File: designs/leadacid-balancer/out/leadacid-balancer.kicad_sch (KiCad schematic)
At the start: 0 parts

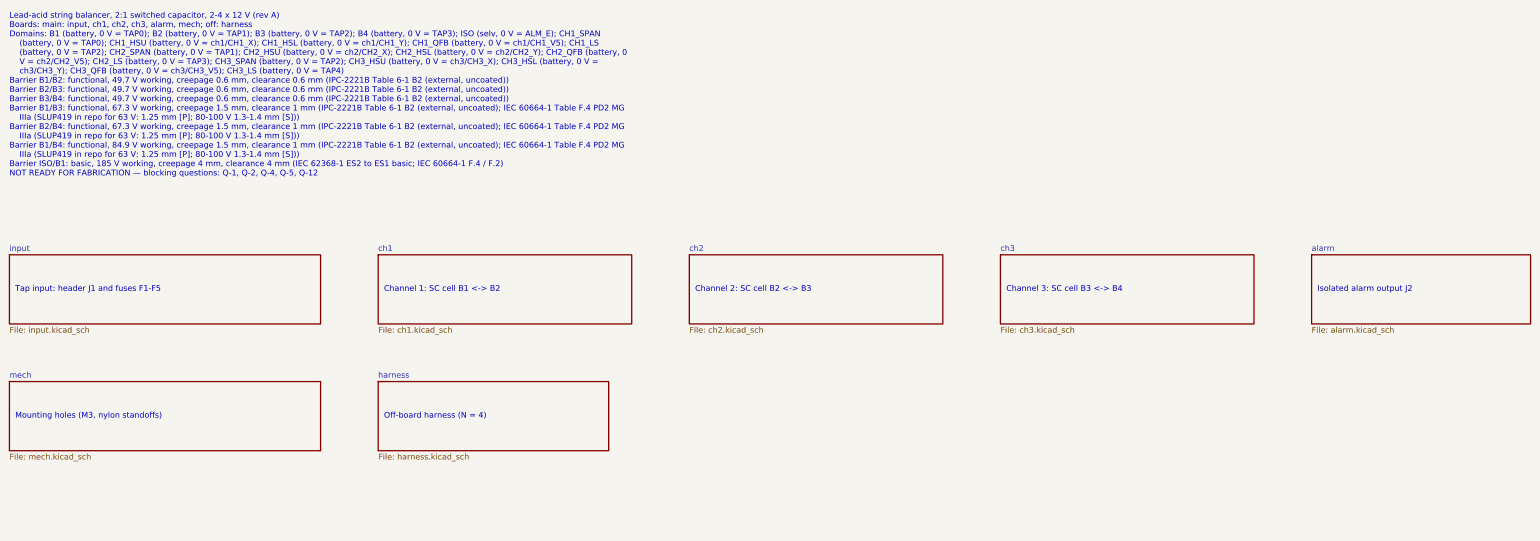
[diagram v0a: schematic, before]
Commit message: designs: work-in-progress (review fixes under way)
Co-Authored-By: Claude Opus 5.5 <noreply@anthropic.com>
Claude-Session: https://claude.ai/code/session_01VFJn9VbX8h27kf4LpLwEtn
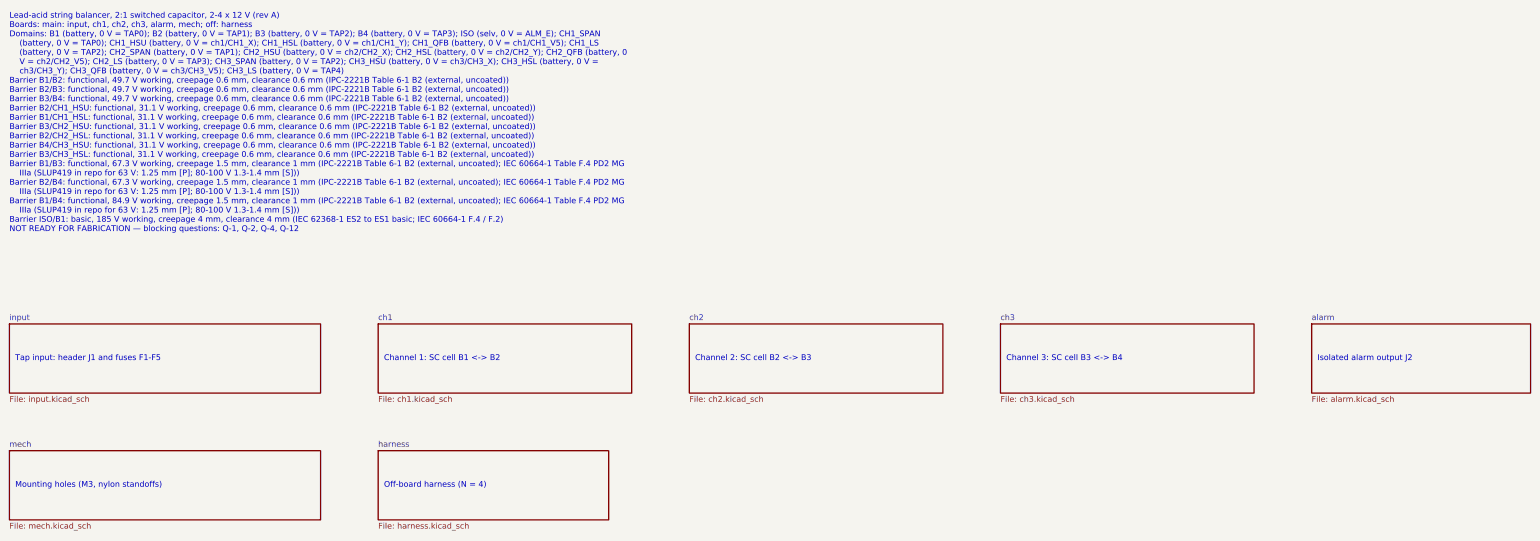
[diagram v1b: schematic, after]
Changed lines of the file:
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@@
 	)
 	(sheet
-		(at 25.4 78.74)
+		(at 25.4 93.98)
 		(size 68.58 15.24)
 		(exclude_from_sim no)
@@
 		)
 		(property "Sheetname" "input"
-			(at 25.4 78.04 0)
+			(at 25.4 93.28 0)
 			(effects
 				(font (size 1.27 1.27))
@@
 		)
 		(property "Sheetfile" "input.kicad_sch"
-			(at 25.4 94.58 0)
+			(at 25.4 109.82 0)
 			(effects
 				(font (size 1.27 1.27))
@@
 	(text "Tap input: header J1 and fuses F1-F5"
 		(exclude_from_sim no)
-		(at 26.67 86.36 0)
-		(effects
-			(font (size 1.27 1.27))
-			(justify left)
-		)
-	)
-	(sheet
-		(at 106.68 78.74)
+		(at 26.67 101.6 0)
+		(effects
+			(font (size 1.27 1.27))
+			(justify left)
+		)
+	)
+	(sheet
+		(at 106.68 93.98)
 		(size 55.88 15.24)
 		(exclude_from_sim no)
@@
 		)
 		(property "Sheetname" "ch1"
-			(at 106.68 78.04 0)
+			(at 106.68 93.28 0)
 			(effects
 				(font (size 1.27 1.27))
@@
 		)
 		(property "Sheetfile" "ch1.kicad_sch"
-			(at 106.68 94.58 0)
+			(at 106.68 109.82 0)
 			(effects
 				(font (size 1.27 1.27))
@@
 	(text "Channel 1: SC cell B1 <-> B2"
 		(exclude_from_sim no)
-		(at 107.95 86.36 0)
-		(effects
-			(font (size 1.27 1.27))
-			(justify left)
-		)
-	)
-	(sheet
-		(at 175.26 78.74)
+		(at 107.95 101.6 0)
+		(effects
+			(font (size 1.27 1.27))
+			(justify left)
+		)
+	)
+	(sheet
+		(at 175.26 93.98)
 		(size 55.88 15.24)
 		(exclude_from_sim no)
@@
 		)
 		(property "Sheetname" "ch2"
-			(at 175.26 78.04 0)
+			(at 175.26 93.28 0)
 			(effects
 				(font (size 1.27 1.27))
@@
 		)
 		(property "Sheetfile" "ch2.kicad_sch"
-			(at 175.26 94.58 0)
+			(at 175.26 109.82 0)
 			(effects
 				(font (size 1.27 1.27))
@@
 	(text "Channel 2: SC cell B2 <-> B3"
 		(exclude_from_sim no)
-		(at 176.53 86.36 0)
-		(effects
-			(font (size 1.27 1.27))
-			(justify left)
-		)
-	)
-	(sheet
-		(at 243.84 78.74)
+		(at 176.53 101.6 0)
+		(effects
+			(font (size 1.27 1.27))
+			(justify left)
+		)
+	)
+	(sheet
+		(at 243.84 93.98)
 		(size 55.88 15.24)
 		(exclude_from_sim no)
@@
 		)
 		(property "Sheetname" "ch3"
-			(at 243.84 78.04 0)
+			(at 243.84 93.28 0)
 			(effects
 				(font (size 1.27 1.27))
@@
 		)
 		(property "Sheetfile" "ch3.kicad_sch"
-			(at 243.84 94.58 0)
+			(at 243.84 109.82 0)
 			(effects
 				(font (size 1.27 1.27))
@@
 	(text "Channel 3: SC cell B3 <-> B4"
 		(exclude_from_sim no)
-		(at 245.11 86.36 0)
-		(effects
-			(font (size 1.27 1.27))
-			(justify left)
-		)
-	)
-	(sheet
-		(at 312.42 78.74)
+		(at 245.11 101.6 0)
+		(effects
+			(font (size 1.27 1.27))
+			(justify left)
+		)
+	)
+	(sheet
+		(at 312.42 93.98)
 		(size 48.26 15.24)
 		(exclude_from_sim no)
@@
 		)
 		(property "Sheetname" "alarm"
-			(at 312.42 78.04 0)
+			(at 312.42 93.28 0)
 			(effects
 				(font (size 1.27 1.27))
@@
 		)
 		(property "Sheetfile" "alarm.kicad_sch"
-			(at 312.42 94.58 0)
+			(at 312.42 109.82 0)
 			(effects
 				(font (size 1.27 1.27))
@@
 	(text "Isolated alarm output J2"
 		(exclude_from_sim no)
-		(at 313.69 86.36 0)
-		(effects
-			(font (size 1.27 1.27))
-			(justify left)
-		)
-	)
-	(sheet
-		(at 25.4 106.68)
+		(at 313.69 101.6 0)
+		(effects
+			(font (size 1.27 1.27))
+			(justify left)
+		)
+	)
+	(sheet
+		(at 25.4 121.92)
 		(size 68.58 15.24)
 		(exclude_from_sim no)
@@
 		)
 		(property "Sheetname" "mech"
-			(at 25.4 105.98 0)
+			(at 25.4 121.22 0)
 			(effects
 				(font (size 1.27 1.27))
@@
 		)
 		(property "Sheetfile" "mech.kicad_sch"
-			(at 25.4 122.52 0)
+			(at 25.4 137.76 0)
 			(effects
 				(font (size 1.27 1.27))
@@
 	(text "Mounting holes (M3, nylon standoffs)"
 		(exclude_from_sim no)
-		(at 26.67 114.3 0)
-		(effects
-			(font (size 1.27 1.27))
-			(justify left)
-		)
-	)
-	(sheet
-		(at 106.68 106.68)
+		(at 26.67 129.54 0)
+		(effects
+			(font (size 1.27 1.27))
+			(justify left)
+		)
+	)
+	(sheet
+		(at 106.68 121.92)
 		(size 50.8 15.24)
 		(exclude_from_sim no)
@@
 		)
 		(property "Sheetname" "harness"
-			(at 106.68 105.98 0)
+			(at 106.68 121.22 0)
 			(effects
 				(font (size 1.27 1.27))
@@
 		)
 		(property "Sheetfile" "harness.kicad_sch"
-			(at 106.68 122.52 0)
+			(at 106.68 137.76 0)
 			(effects
 				(font (size 1.27 1.27))
@@
 	(text "Off-board harness (N = 4)"
 		(exclude_from_sim no)
-		(at 107.95 114.3 0)
-		(effects
-			(font (size 1.27 1.27))
-			(justify left)
-		)
-	)
-	(text "Lead-acid string balancer, 2:1 switched capacitor, 2-4 x 12 V (rev A)\nBoards: main: input, ch1, ch2, ch3, alarm, mech; off: harness\nDomains: B1 (battery, 0 V = TAP0); B2 (battery, 0 V = TAP1); B3 (battery, 0 V = TAP2); B4 (battery, 0 V = TAP3); ISO (selv, 0 V = ALM_E); CH1_SPAN\n    (battery, 0 V = TAP0); CH1_HSU (battery, 0 V = ch1/CH1_X); CH1_HSL (battery, 0 V = ch1/CH1_Y); CH1_QFB (battery, 0 V = ch1/CH1_V5); CH1_LS\n    (battery, 0 V = TAP2); CH2_SPAN (battery, 0 V = TAP1); CH2_HSU (battery, 0 V = ch2/CH2_X); CH2_HSL (battery, 0 V = ch2/CH2_Y); CH2_QFB (battery, 0\n    V = ch2/CH2_V5); CH2_LS (battery, 0 V = TAP3); CH3_SPAN (battery, 0 V = TAP2); CH3_HSU (battery, 0 V = ch3/CH3_X); CH3_HSL (battery, 0 V =\n    ch3/CH3_Y); CH3_QFB (battery, 0 V = ch3/CH3_V5); CH3_LS (battery, 0 V = TAP4)\nBarrier B1/B2: functional, 49.7 V working, creepage 0.6 mm, clearance 0.6 mm (IPC-2221B Table 6-1 B2 (external, uncoated))\nBarrier B2/B3: functional, 49.7 V working, creepage 0.6 mm, clearance 0.6 mm (IPC-2221B Table 6-1 B2 (external, uncoated))\nBarrier B3/B4: functional, 49.7 V working, creepage 0.6 mm, clearance 0.6 mm (IPC-2221B Table 6-1 B2 (external, uncoated))\nBarrier B1/B3: functional, 67.3 V working, creepage 1.5 mm, clearance 1 mm (IPC-2221B Table 6-1 B2 (external, uncoated); IEC 60664-1 Table F.4 PD2 MG\n    IIIa (SLUP419 in repo for 63 V: 1.25 mm [P]; 80-100 V 1.3-1.4 mm [S]))\nBarrier B2/B4: functional, 67.3 V working, creepage 1.5 mm, clearance 1 mm (IPC-2221B Table 6-1 B2 (external, uncoated); IEC 60664-1 Table F.4 PD2 MG\n    IIIa (SLUP419 in repo for 63 V: 1.25 mm [P]; 80-100 V 1.3-1.4 mm [S]))\nBarrier B1/B4: functional, 84.9 V working, creepage 1.5 mm, clearance 1 mm (IPC-2221B Table 6-1 B2 (external, uncoated); IEC 60664-1 Table F.4 PD2 MG\n    IIIa (SLUP419 in repo for 63 V: 1.25 mm [P]; 80-100 V 1.3-1.4 mm [S]))\nBarrier ISO/B1: basic, 185 V working, creepage 4 mm, clearance 4 mm (IEC 62368-1 ES2 to ES1 basic; IEC 60664-1 F.4 / F.2)\nNOT READY FOR FABRICATION — blocking questions: Q-1, Q-2, Q-4, Q-5, Q-12"
+		(at 107.95 129.54 0)
+		(effects
+			(font (size 1.27 1.27))
+			(justify left)
+		)
+	)
+	(text "Lead-acid string balancer, 2:1 switched capacitor, 2-4 x 12 V (rev A)\nBoards: main: input, ch1, ch2, ch3, alarm, mech; off: harness\nDomains: B1 (battery, 0 V = TAP0); B2 (battery, 0 V = TAP1); B3 (battery, 0 V = TAP2); B4 (battery, 0 V = TAP3); ISO (selv, 0 V = ALM_E); CH1_SPAN\n    (battery, 0 V = TAP0); CH1_HSU (battery, 0 V = ch1/CH1_X); CH1_HSL (battery, 0 V = ch1/CH1_Y); CH1_QFB (battery, 0 V = ch1/CH1_V5); CH1_LS\n    (battery, 0 V = TAP2); CH2_SPAN (battery, 0 V = TAP1); CH2_HSU (battery, 0 V = ch2/CH2_X); CH2_HSL (battery, 0 V = ch2/CH2_Y); CH2_QFB (battery, 0\n    V = ch2/CH2_V5); CH2_LS (battery, 0 V = TAP3); CH3_SPAN (battery, 0 V = TAP2); CH3_HSU (battery, 0 V = ch3/CH3_X); CH3_HSL (battery, 0 V =\n    ch3/CH3_Y); CH3_QFB (battery, 0 V = ch3/CH3_V5); CH3_LS (battery, 0 V = TAP4)\nBarrier B1/B2: functional, 49.7 V working, creepage 0.6 mm, clearance 0.6 mm (IPC-2221B Table 6-1 B2 (external, uncoated))\nBarrier B2/B3: functional, 49.7 V working, creepage 0.6 mm, clearance 0.6 mm (IPC-2221B Table 6-1 B2 (external, uncoated))\nBarrier B3/B4: functional, 49.7 V working, creepage 0.6 mm, clearance 0.6 mm (IPC-2221B Table 6-1 B2 (external, uncoated))\nBarrier B2/CH1_HSU: functional, 31.1 V working, creepage 0.6 mm, clearance 0.6 mm (IPC-2221B Table 6-1 B2 (external, uncoated))\nBarrier B1/CH1_HSL: functional, 31.1 V working, creepage 0.6 mm, clearance 0.6 mm (IPC-2221B Table 6-1 B2 (external, uncoated))\nBarrier B3/CH2_HSU: functional, 31.1 V working, creepage 0.6 mm, clearance 0.6 mm (IPC-2221B Table 6-1 B2 (external, uncoated))\nBarrier B2/CH2_HSL: functional, 31.1 V working, creepage 0.6 mm, clearance 0.6 mm (IPC-2221B Table 6-1 B2 (external, uncoated))\nBarrier B4/CH3_HSU: functional, 31.1 V working, creepage 0.6 mm, clearance 0.6 mm (IPC-2221B Table 6-1 B2 (external, uncoated))\nBarrier B3/CH3_HSL: functional, 31.1 V working, creepage 0.6 mm, clearance 0.6 mm (IPC-2221B Table 6-1 B2 (external, uncoated))\nBarrier B1/B3: functional, 67.3 V working, creepage 1.5 mm, clearance 1 mm (IPC-2221B Table 6-1 B2 (external, uncoated); IEC 60664-1 Table F.4 PD2 MG\n    IIIa (SLUP419 in repo for 63 V: 1.25 mm [P]; 80-100 V 1.3-1.4 mm [S]))\nBarrier B2/B4: functional, 67.3 V working, creepage 1.5 mm, clearance 1 mm (IPC-2221B Table 6-1 B2 (external, uncoated); IEC 60664-1 Table F.4 PD2 MG\n    IIIa (SLUP419 in repo for 63 V: 1.25 mm [P]; 80-100 V 1.3-1.4 mm [S]))\nBarrier B1/B4: functional, 84.9 V working, creepage 1.5 mm, clearance 1 mm (IPC-2221B Table 6-1 B2 (external, uncoated); IEC 60664-1 Table F.4 PD2 MG\n    IIIa (SLUP419 in repo for 63 V: 1.25 mm [P]; 80-100 V 1.3-1.4 mm [S]))\nBarrier ISO/B1: basic, 185 V working, creepage 4 mm, clearance 4 mm (IEC 62368-1 ES2 to ES1 basic; IEC 60664-1 F.4 / F.2)\nNOT READY FOR FABRICATION — blocking questions: Q-1, Q-2, Q-4, Q-12"
 		(exclude_from_sim no)
 		(at 25.4 25.4 0)
